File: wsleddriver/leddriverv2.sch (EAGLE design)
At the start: 18 parts, among them IC1 WS2811-SOP8, X3 TSW-103-07-G-S, X4 TSW-103-07-G-S

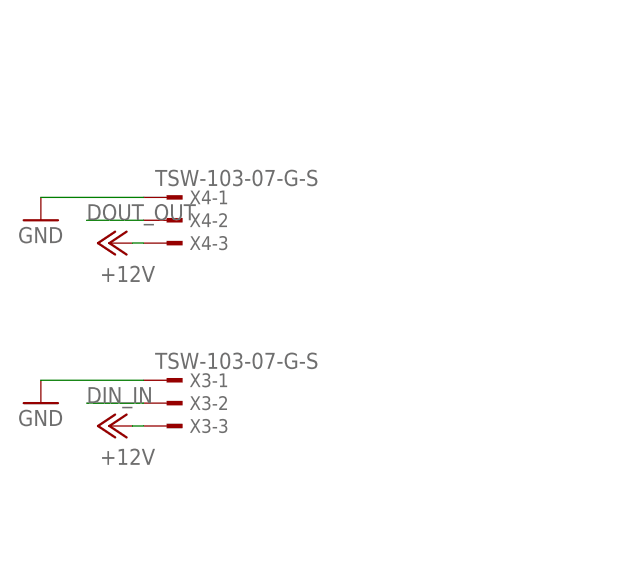
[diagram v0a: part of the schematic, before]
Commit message: w
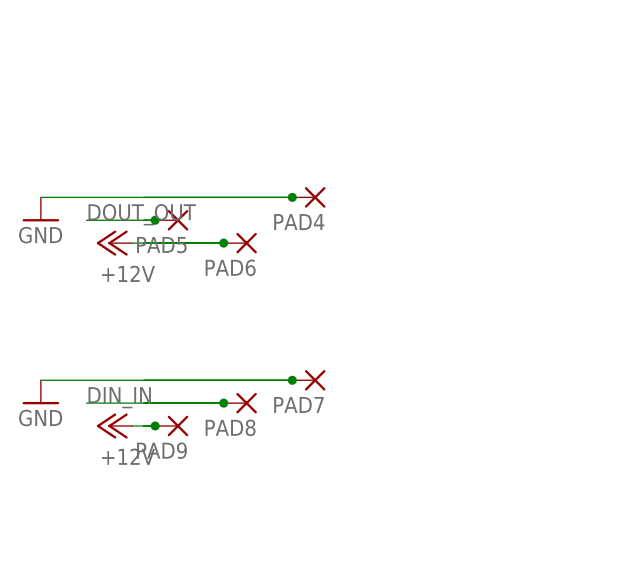
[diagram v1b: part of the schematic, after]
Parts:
- removed X3, X4: TSW-103-07-G-S, con-samtec:TSW-103-07-G-S
- added PAD4, PAD5, PAD6, PAD7, PAD8, PAD9: (no value), wirepad:2,54/1,1
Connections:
- net +12V: now also PAD6.P, PAD9.P; no longer X3-3.1, X4-3.1
- net DIN_IN: now also PAD8.P; no longer X3-2.1
- net DOUT_OUT: now also PAD5.P; no longer X4-2.1
- net GND: now also PAD4.P, PAD7.P; no longer X3-1.1, X4-1.1
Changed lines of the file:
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@@
 <?xml version="1.0" encoding="utf-8"?>
 <!DOCTYPE eagle SYSTEM "eagle.dtd">
-<eagle version="9.2.2">
+<eagle version="9.4.2">
 <drawing>
 <settings>
@@
 <part name="PAD2" library="wirepad" library_urn="urn:adsk.eagle:library:412" deviceset="3,81/1,4" device="" package3d_urn="urn:adsk.eagle:package:30835/1"/>
 <part name="PAD3" library="wirepad" library_urn="urn:adsk.eagle:library:412" deviceset="3,81/1,4" device="" package3d_urn="urn:adsk.eagle:package:30835/1"/>
-<part name="X3" library="con-samtec" library_urn="urn:adsk.eagle:library:184" deviceset="TSW-103-*-G-S" device="" technology="07"/>
-<part name="X4" library="con-samtec" library_urn="urn:adsk.eagle:library:184" deviceset="TSW-103-*-G-S" device="" technology="07"/>
 <part name="GND1" library="supply1" library_urn="urn:adsk.eagle:library:371" deviceset="GND" device=""/>
 <part name="GND2" library="supply1" library_urn="urn:adsk.eagle:library:371" deviceset="GND" device=""/>
 <part name="P+1" library="supply1" library_urn="urn:adsk.eagle:library:371" deviceset="+12V" device=""/>
 <part name="P+2" library="supply1" library_urn="urn:adsk.eagle:library:371" deviceset="+12V" device=""/>
+<part name="PAD4" library="wirepad" library_urn="urn:adsk.eagle:library:412" deviceset="2,54/1,1" device="" package3d_urn="urn:adsk.eagle:package:30836/1"/>
+<part name="PAD5" library="wirepad" library_urn="urn:adsk.eagle:library:412" deviceset="2,54/1,1" device="" package3d_urn="urn:adsk.eagle:package:30836/1"/>
+<part name="PAD6" library="wirepad" library_urn="urn:adsk.eagle:library:412" deviceset="2,54/1,1" device="" package3d_urn="urn:adsk.eagle:package:30836/1"/>
+<part name="PAD7" library="wirepad" library_urn="urn:adsk.eagle:library:412" deviceset="2,54/1,1" device="" package3d_urn="urn:adsk.eagle:package:30836/1"/>
+<part name="PAD8" library="wirepad" library_urn="urn:adsk.eagle:library:412" deviceset="2,54/1,1" device="" package3d_urn="urn:adsk.eagle:package:30836/1"/>
+<part name="PAD9" library="wirepad" library_urn="urn:adsk.eagle:library:412" deviceset="2,54/1,1" device="" package3d_urn="urn:adsk.eagle:package:30836/1"/>
 </parts>
 <sheets>
@@
 <attribute name="VALUE" x="16.637" y="19.558" size="1.778" layer="96"/>
 </instance>
-<instance part="X3" gate="-1" x="-85.09" y="40.64" smashed="yes">
-<attribute name="VALUE" x="-86.36" y="41.91" size="1.778" layer="96"/>
-<attribute name="NAME" x="-82.55" y="39.878" size="1.524" layer="95"/>
-</instance>
-<instance part="X3" gate="-2" x="-85.09" y="38.1" smashed="yes">
-<attribute name="NAME" x="-82.55" y="37.338" size="1.524" layer="95"/>
-</instance>
-<instance part="X3" gate="-3" x="-85.09" y="35.56" smashed="yes">
-<attribute name="NAME" x="-82.55" y="34.798" size="1.524" layer="95"/>
-</instance>
-<instance part="X4" gate="-1" x="-85.09" y="60.96" smashed="yes">
-<attribute name="VALUE" x="-86.36" y="62.23" size="1.778" layer="96"/>
-<attribute name="NAME" x="-82.55" y="60.198" size="1.524" layer="95"/>
-</instance>
-<instance part="X4" gate="-2" x="-85.09" y="58.42" smashed="yes">
-<attribute name="NAME" x="-82.55" y="57.658" size="1.524" layer="95"/>
-</instance>
-<instance part="X4" gate="-3" x="-85.09" y="55.88" smashed="yes">
-<attribute name="NAME" x="-82.55" y="55.118" size="1.524" layer="95"/>
-</instance>
 <instance part="GND1" gate="1" x="-99.06" y="58.42" smashed="yes">
 <attribute name="VALUE" x="-101.6" y="55.88" size="1.778" layer="96"/>
@@
 <instance part="P+2" gate="1" x="-91.44" y="55.88" smashed="yes" rot="R90">
 <attribute name="VALUE" x="-86.36" y="53.34" size="1.778" layer="96" rot="R180"/>
+</instance>
+<instance part="PAD4" gate="1" x="-68.58" y="60.96" smashed="yes" rot="R180">
+<attribute name="NAME" x="-67.437" y="59.1058" size="1.778" layer="95" rot="R180"/>
+<attribute name="VALUE" x="-67.437" y="64.262" size="1.778" layer="96" rot="R180"/>
+</instance>
+<instance part="PAD5" gate="1" x="-83.82" y="58.42" smashed="yes" rot="R180">
+<attribute name="NAME" x="-82.677" y="56.5658" size="1.778" layer="95" rot="R180"/>
+<attribute name="VALUE" x="-82.677" y="61.722" size="1.778" layer="96" rot="R180"/>
+</instance>
+<instance part="PAD6" gate="1" x="-76.2" y="55.88" smashed="yes" rot="R180">
+<attribute name="NAME" x="-75.057" y="54.0258" size="1.778" layer="95" rot="R180"/>
+<attribute name="VALUE" x="-75.057" y="59.182" size="1.778" layer="96" rot="R180"/>
+</instance>
+<instance part="PAD7" gate="1" x="-68.58" y="40.64" smashed="yes" rot="R180">
+<attribute name="NAME" x="-67.437" y="38.7858" size="1.778" layer="95" rot="R180"/>
+<attribute name="VALUE" x="-67.437" y="43.942" size="1.778" layer="96" rot="R180"/>
+</instance>
+<instance part="PAD8" gate="1" x="-76.2" y="38.1" smashed="yes" rot="R180">
+<attribute name="NAME" x="-75.057" y="36.2458" size="1.778" layer="95" rot="R180"/>
+<attribute name="VALUE" x="-75.057" y="41.402" size="1.778" layer="96" rot="R180"/>
+</instance>
+<instance part="PAD9" gate="1" x="-83.82" y="35.56" smashed="yes" rot="R180">
+<attribute name="NAME" x="-82.677" y="33.7058" size="1.778" layer="95" rot="R180"/>
+<attribute name="VALUE" x="-82.677" y="38.862" size="1.778" layer="96" rot="R180"/>
 </instance>
 </instances>
@@
 </segment>
 <segment>
-<pinref part="X4" gate="-3" pin="1"/>
 <pinref part="P+2" gate="1" pin="+12V"/>
-<wire x1="-87.63" y1="55.88" x2="-88.9" y2="55.88" width="0.1524" layer="91"/>
-</segment>
-<segment>
-<pinref part="X3" gate="-3" pin="1"/>
+<wire x1="-87.63" y1="55.88" x2="-78.74" y2="55.88" width="0.1524" layer="91"/>
+<pinref part="PAD6" gate="1" pin="P"/>
+<junction x="-78.74" y="55.88"/>
+<wire x1="-78.74" y1="55.88" x2="-88.9" y2="55.88" width="0.1524" layer="91"/>
+</segment>
+<segment>
 <pinref part="P+1" gate="1" pin="+12V"/>
-<wire x1="-87.63" y1="35.56" x2="-88.9" y2="35.56" width="0.1524" layer="91"/>
+<wire x1="-87.63" y1="35.56" x2="-86.36" y2="35.56" width="0.1524" layer="91"/>
+<pinref part="PAD9" gate="1" pin="P"/>
+<junction x="-86.36" y="35.56"/>
+<wire x1="-86.36" y1="35.56" x2="-88.9" y2="35.56" width="0.1524" layer="91"/>
 </segment>
 </net>
@@
 <segment>
 <pinref part="GND1" gate="1" pin="GND"/>
-<wire x1="-99.06" y1="60.96" x2="-87.63" y2="60.96" width="0.1524" layer="91"/>
-<pinref part="X4" gate="-1" pin="1"/>
-</segment>
-<segment>
-<pinref part="X3" gate="-1" pin="1"/>
+<wire x1="-99.06" y1="60.96" x2="-71.12" y2="60.96" width="0.1524" layer="91"/>
+<pinref part="PAD4" gate="1" pin="P"/>
+<wire x1="-71.12" y1="60.96" x2="-87.63" y2="60.96" width="0.1524" layer="91"/>
+<junction x="-71.12" y="60.96"/>
+</segment>
+<segment>
 <pinref part="GND2" gate="1" pin="GND"/>
-<wire x1="-87.63" y1="40.64" x2="-99.06" y2="40.64" width="0.1524" layer="91"/>
+<wire x1="-87.63" y1="40.64" x2="-71.12" y2="40.64" width="0.1524" layer="91"/>
+<pinref part="PAD7" gate="1" pin="P"/>
+<wire x1="-71.12" y1="40.64" x2="-99.06" y2="40.64" width="0.1524" layer="91"/>
+<junction x="-71.12" y="40.64"/>
 </segment>
 </net>
@@
 </segment>
 <segment>
-<pinref part="X3" gate="-2" pin="1"/>
-<wire x1="-87.63" y1="38.1" x2="-93.98" y2="38.1" width="0.1524" layer="91"/>
+<wire x1="-87.63" y1="38.1" x2="-78.74" y2="38.1" width="0.1524" layer="91"/>
 <label x="-93.98" y="38.1" size="1.778" layer="95"/>
+<pinref part="PAD8" gate="1" pin="P"/>
+<wire x1="-78.74" y1="38.1" x2="-93.98" y2="38.1" width="0.1524" layer="91"/>
+<junction x="-78.74" y="38.1"/>
 </segment>
 </net>
@@
 </segment>
 <segment>
-<pinref part="X4" gate="-2" pin="1"/>
-<wire x1="-87.63" y1="58.42" x2="-93.98" y2="58.42" width="0.1524" layer="91"/>
+<wire x1="-87.63" y1="58.42" x2="-86.36" y2="58.42" width="0.1524" layer="91"/>
 <label x="-93.98" y="58.42" size="1.778" layer="95"/>
+<pinref part="PAD5" gate="1" pin="P"/>
+<wire x1="-86.36" y1="58.42" x2="-93.98" y2="58.42" width="0.1524" layer="91"/>
+<junction x="-86.36" y="58.42"/>
 </segment>
 </net>
